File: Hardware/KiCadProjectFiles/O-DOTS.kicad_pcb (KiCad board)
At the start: 2 copper layers, 71.1 x 58.4 mm, 27 parts, among them IC1 ATMEGA328P-P, U1 FQD5P20, U2 DS1337, U3 SerialHeader, U4 RFIDHeader, Y1 Crystal

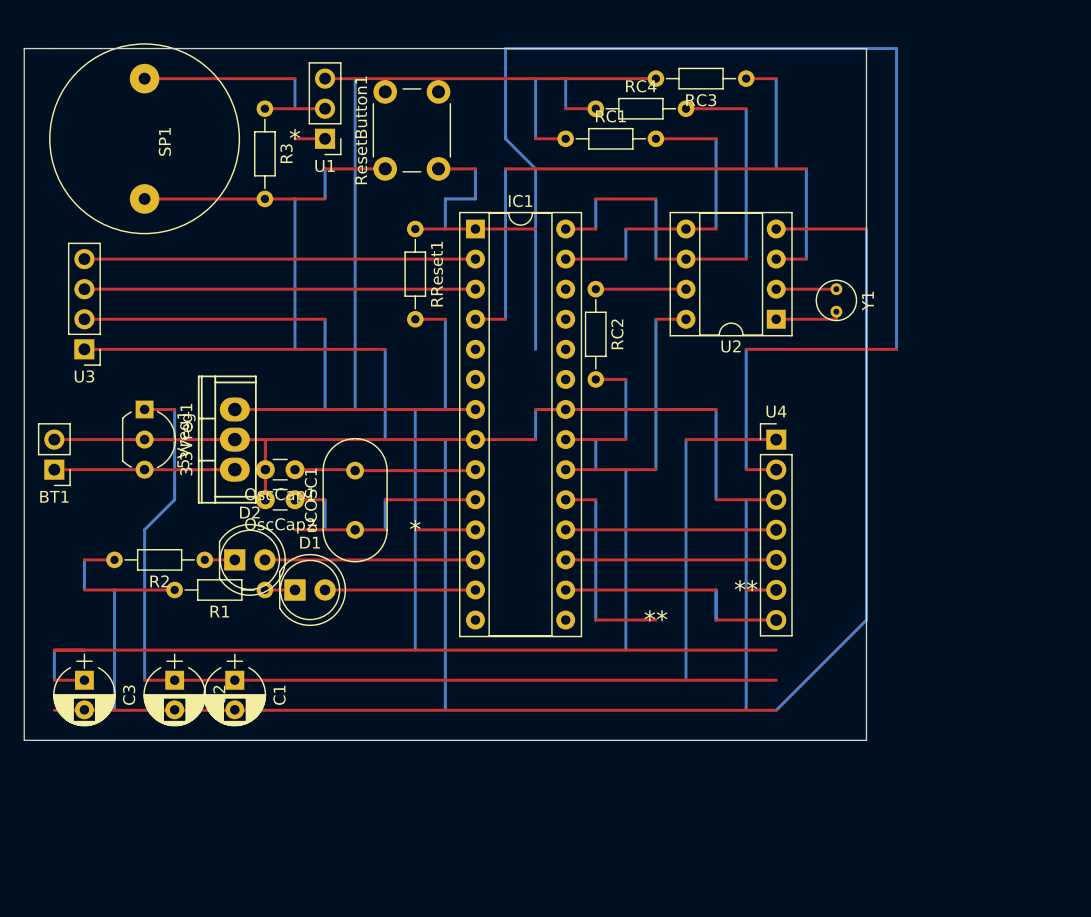
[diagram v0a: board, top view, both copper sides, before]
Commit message: updated pcb stuff
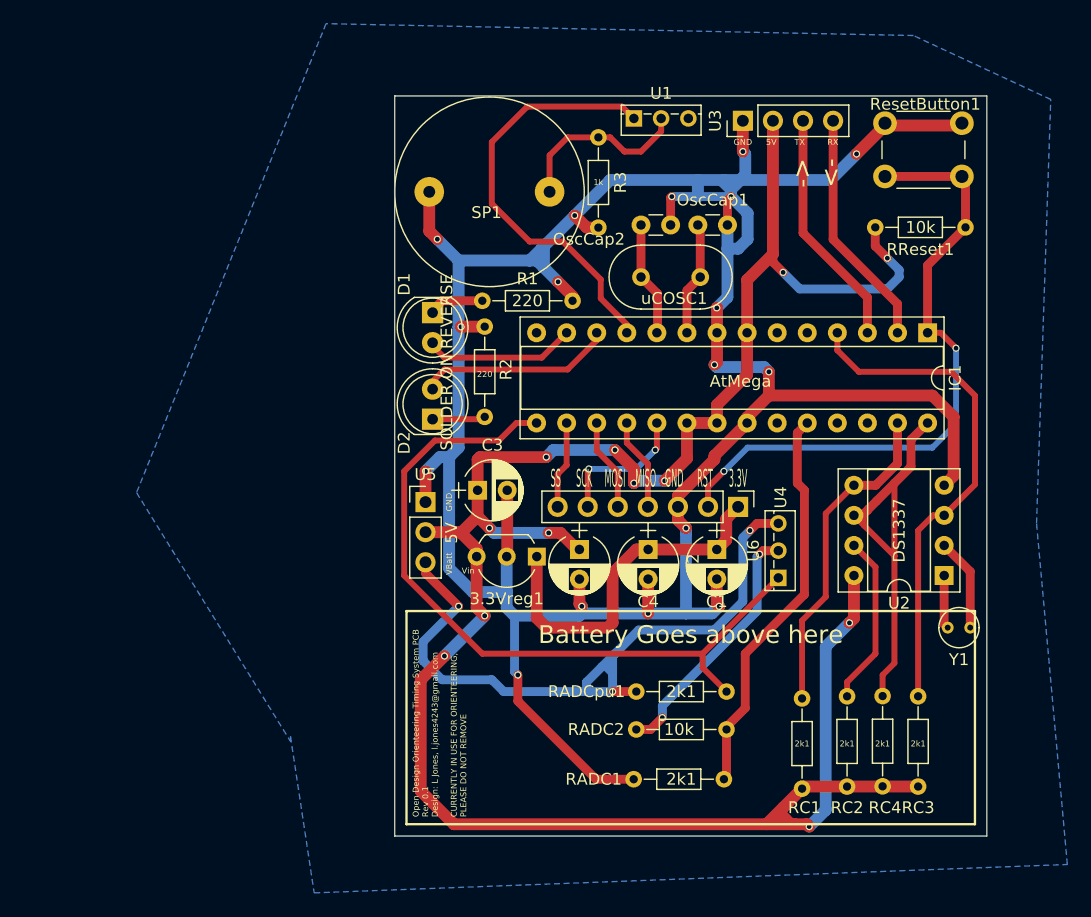
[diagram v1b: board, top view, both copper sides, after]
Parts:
- removed 5Vreg1: L78M05abv, Power_Integrations:TO-220
- removed BT1: Battery, Pin_Headers:Pin_Header_Straight_1x02_Pitch2.54mm
- added C4: 10uF, Capacitors_ThroughHole:CP_Radial_D5.0mm_P2.50mm, F.Cu at (118.0, 105.8)
- added RADC1: 2k1, Resistors_ThroughHole:R_Axial_DIN0204_L3.6mm_D1.6mm_P7.62mm_Horizontal, F.Cu at (130.2, 125.2)
- added RADC2: 10k, Resistors_ThroughHole:R_Axial_DIN0204_L3.6mm_D1.6mm_P7.62mm_Horizontal, F.Cu at (122.8, 121.0)
- added RADCpu1: 2k1, Resistors_ThroughHole:R_Axial_DIN0204_L3.6mm_D1.6mm_P7.62mm_Horizontal, F.Cu at (122.8, 117.8)
- added U5: BatteryInterface, Pin_Headers:Pin_Header_Straight_1x03_Pitch2.54mm, F.Cu at (105.0, 101.8)
- added U6: FQD5P20, TO_SOT_Packages_THT:TO-251_IPAK_Vertical, F.Cu at (134.8, 108.2)
- U1: footprint Pin_Headers:Pin_Header_Straight_1x03_Pitch2.54mm -> TO_SOT_Packages_THT:TO-251_IPAK_Vertical
- moved RC4 62.1 mm to (143.6, 125.8), turned to 90 degrees
- moved U3 58.9 mm to (131.8, 69.6), turned to 90 degrees
- moved RC1 58.4 mm to (136.8, 126.0), turned to 90 degrees
- moved RC3 54.1 mm to (146.6, 118.2), turned to 270 degrees
- moved RReset1 46.5 mm to (150.6, 78.6), turned to 180 degrees
- moved ResetButton1 42.4 mm to (143.8, 69.8), turned to 0 degrees
- moved C1 42.2 mm to (129.6, 105.8)
- moved C2 41.5 mm to (123.8, 105.8)
- moved RC2 40.4 mm to (140.6, 118.2)
- moved OscCap1 39.8 mm to (128.0, 78.4), turned to 0 degrees
- moved IC1 39.2 mm to (147.4, 87.5), turned to 270 degrees
- moved OscCap2 37.3 mm to (123.2, 78.4), turned to 0 degrees
- moved C3 36.9 mm to (109.4, 100.8), turned to 0 degrees
- moved 3.3Vreg1 35.4 mm to (114.4, 106.4), turned to 180 degrees
- moved uCOSC1 32.2 mm to (123.2, 82.8), turned to 0 degrees
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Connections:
- 3.3Vreg1 pad 3: Net-(3.3Vreg1-Pad3) -> 5V
- IC1 pad 22: Net-(IC1-Pad22) -> GND
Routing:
- net (no net): track 640.3 -> 0.00 mm
- net GND: track 114.3 -> 249.8 mm, vias 0 -> 17
- net 5V: track 96.5 -> 190.8 mm, vias 0 -> 12
- net Net-(IC1-Pad15): track 0.00 -> 62.7 mm
- net Net-(RADCpu1-Pad1): track 0.00 -> 60.0 mm, vias 0 -> 3
- net Net-(IC1-Pad1): track 15.8 -> 55.3 mm, vias 0 -> 2
- net Net-(IC1-Pad4): track 7.62 -> 42.6 mm
- net Net-(IC1-Pad24): track 0.00 -> 33.5 mm
- net 3.3V: track 63.5 -> 30.3 mm
- net Net-(IC1-Pad11): track 7.62 -> 36.1 mm
- net Net-(RADC2-Pad1): track 0.00 -> 21.5 mm, vias 0 -> 2
- net Net-(IC1-Pad28): track 15.2 -> 36.1 mm
- net Net-(3.3Vreg1-Pad3): track 15.2 -> 0.00 mm
- net Net-(IC1-Pad22): track 15.2 -> 0.00 mm
- net Net-(IC1-Pad3): track 33.0 -> 20.2 mm
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- added copper zone on B.Cu, net GND
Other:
- board size 71.1 x 58.4 mm -> 50 x 62.5 mm
- board text added: "-> <-"
- board text added: "10k"
- board text added: "1k"
- board text added: "220"
- board text added: "2k1"
- board text added: "3.3V"
- board text added: "5V"
- board text added: "AtMega"
- board text added: "Battery Goes above here"
- board text added: "DS1337"
- board text added: "GND"
- board text added: "MISO"
- board text added: "MOSI"
- board text added: "Open Design Orienteering Timing System PCB Rev 0.1 Design: L Jones, l.jones4243@gmail.com CURRENTLY IN USE FOR ORIENTEERING, PLEASE DO NOT REMOVE"
- board text added: "RST"
- board text added: "RX"
- board text added: "SCK"
- board text added: "SOLDER ON REVERSE"
- board text added: "SS"
- board text added: "TX"
- board text added: "VBatt"
- board text added: "Vin"
- board text removed: "*"
- board text removed: "**"
- board text removed: "***"
